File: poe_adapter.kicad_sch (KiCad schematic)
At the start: 12 parts

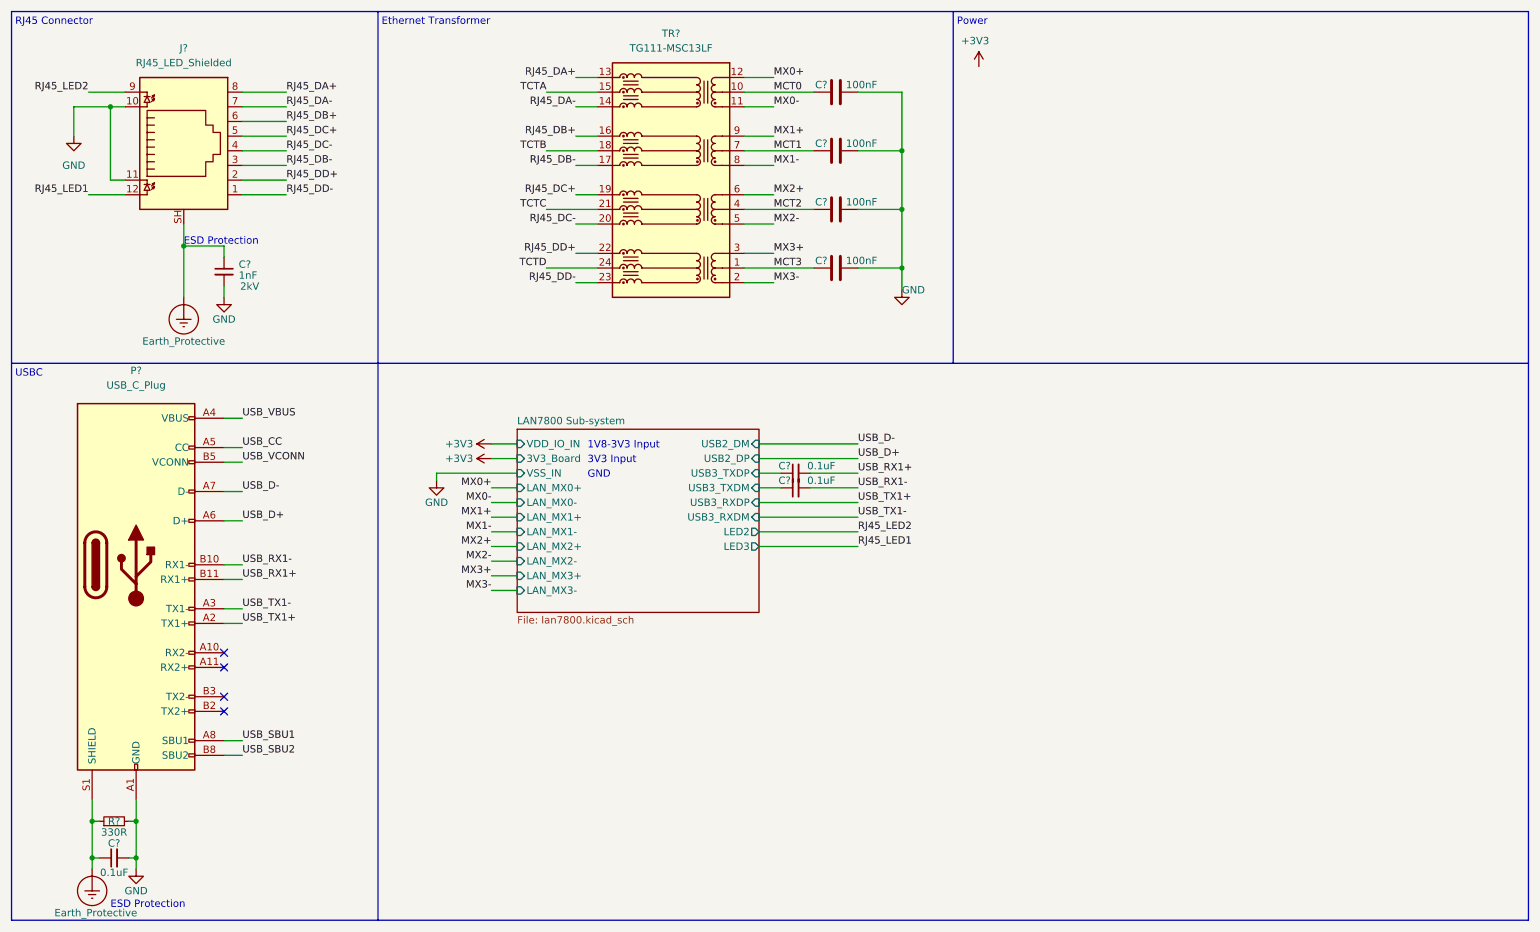
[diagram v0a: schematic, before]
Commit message: led update
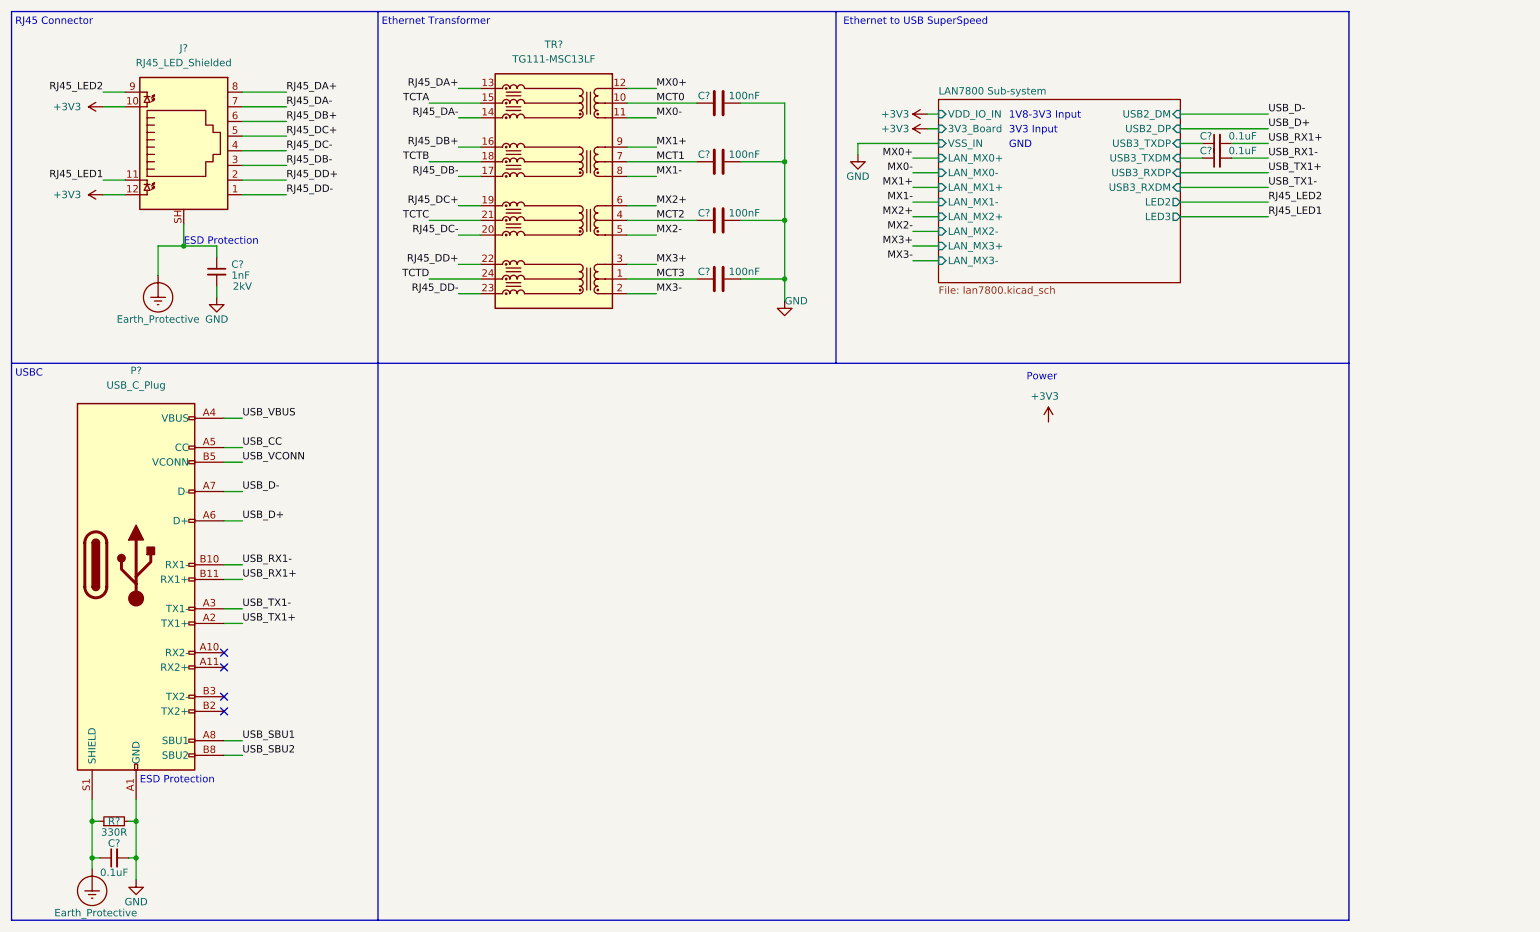
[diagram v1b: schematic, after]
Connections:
- net +3V3: now also J?.10, J?.12
- net GND: no longer J?.10, J?.11
- net RJ45_LED1: now also J?.11; no longer J?.12
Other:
- note added: "Ethernet to USB SuperSpeed"
- moved on the sheet: C?, TR?
